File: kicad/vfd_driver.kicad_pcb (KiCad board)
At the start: 2 copper layers, 181.6 x 35.3 mm, 48 parts, among them CON1 AVR-ISP-6, J1 PWR, J2 Display, J6 MH, J7 MH, J8 MH, J9 MH, U1 ATTINY2313-20SU, U10 74HC595, U11 74HC595, U12 74HC595, U13 74HC595, U14 ULN2803A, U15 ULN2803A, U16 ULN2003, U17 ULN2003, U18 LM1117-3.3, U19 LT1073, U2 74HC595, U3 74HC595, U4 74HC595, U5 74HC595, U6 ULN2803A, U7 ULN2003, U8 ULN2003, U9 ULN2003

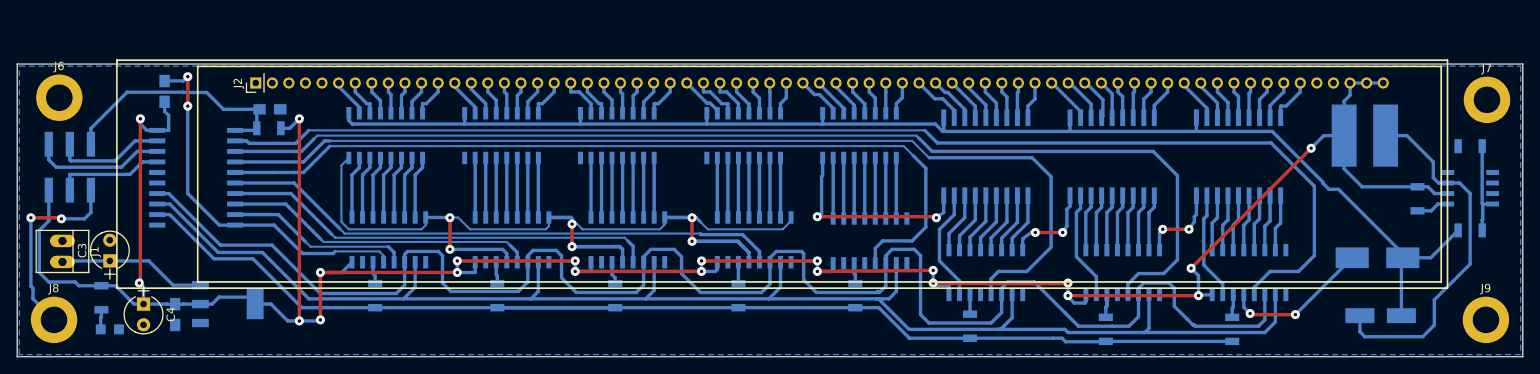
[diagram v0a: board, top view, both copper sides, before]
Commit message: routing
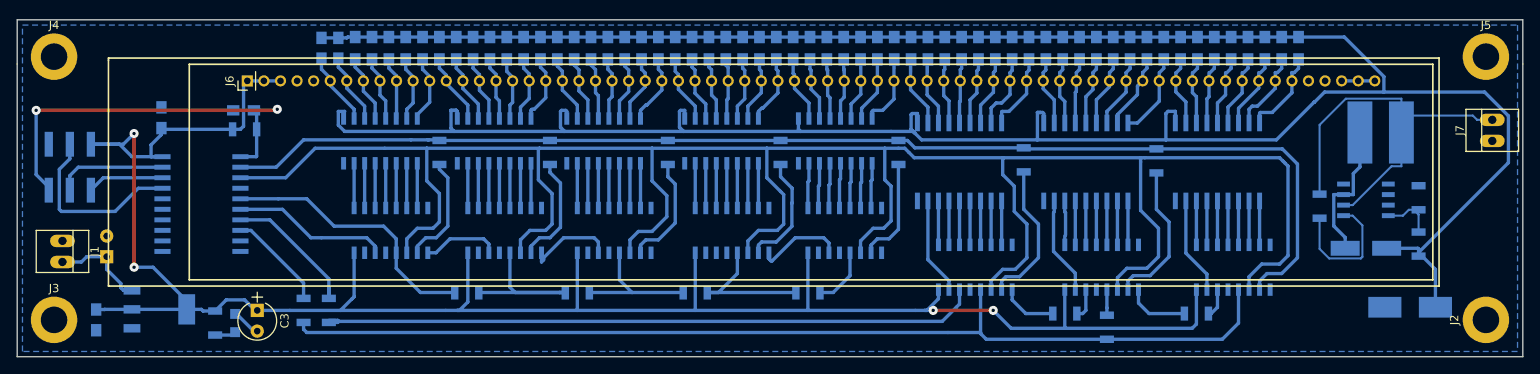
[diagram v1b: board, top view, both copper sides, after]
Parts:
- removed J8, J9: MH, Mounting_Holes:MountingHole_3.2mm_M3_DIN965_Pad
- removed U1: ATTINY2313-20SU, Housings_SOIC:SOIC-20W_7.5x12.8mm_Pitch1.27mm
- removed U2, U3, U4: 74HC595, Housings_SOIC:SOIC-16_3.9x9.9mm_Pitch1.27mm
- added J3: MH, Mounting_Holes:MountingHole_3.2mm_M3_DIN965_Pad, F.Cu at (19.1, 49.5)
- added J4: MH, Mounting_Holes:MountingHole_3.2mm_M3_DIN965_Pad, F.Cu at (19.1, 17.8)
- added J5: MH, Mounting_Holes:MountingHole_3.2mm_M3_DIN965_Pad, F.Cu at (191.8, 17.8)
- added R16: 1k, Resistors_SMD:R_0805_HandSoldering, B.Cu at (55.4, 16.8)
- added R17: 1k, Resistors_SMD:R_0805_HandSoldering, B.Cu at (57.4, 16.8)
- added R18: 1k, Resistors_SMD:R_0805_HandSoldering, B.Cu at (59.4, 16.8)
- added R19: 1k, Resistors_SMD:R_0805_HandSoldering, B.Cu at (61.5, 16.8)
- added R20: 1k, Resistors_SMD:R_0805_HandSoldering, B.Cu at (63.5, 16.8)
- added R21: 1k, Resistors_SMD:R_0805_HandSoldering, B.Cu at (65.5, 16.8)
- added R22: 1k, Resistors_SMD:R_0805_HandSoldering, B.Cu at (67.6, 16.8)
- added R23: 1k, Resistors_SMD:R_0805_HandSoldering, B.Cu at (69.6, 16.8)
- added R24: 1k, Resistors_SMD:R_0805_HandSoldering, B.Cu at (71.6, 16.8)
- added R25: 1k, Resistors_SMD:R_0805_HandSoldering, B.Cu at (73.7, 16.8)
- added R26: 1k, Resistors_SMD:R_0805_HandSoldering, B.Cu at (75.7, 16.8)
- added R27: 1k, Resistors_SMD:R_0805_HandSoldering, B.Cu at (77.7, 16.8)
- added R28: 1k, Resistors_SMD:R_0805_HandSoldering, B.Cu at (79.8, 16.8)
- added R29: 1k, Resistors_SMD:R_0805_HandSoldering, B.Cu at (81.8, 16.8)
- added R30: 1k, Resistors_SMD:R_0805_HandSoldering, B.Cu at (83.8, 16.8)
- added R31: 1k, Resistors_SMD:R_0805_HandSoldering, B.Cu at (85.9, 16.8)
- added R32: 1k, Resistors_SMD:R_0805_HandSoldering, B.Cu at (87.9, 16.8)
- added R33: 1k, Resistors_SMD:R_0805_HandSoldering, B.Cu at (89.9, 16.8)
- added R34: 1k, Resistors_SMD:R_0805_HandSoldering, B.Cu at (91.9, 16.8)
- added R35: 1k, Resistors_SMD:R_0805_HandSoldering, B.Cu at (94.0, 16.8)
- added R36: 1k, Resistors_SMD:R_0805_HandSoldering, B.Cu at (96.0, 16.8)
- added R37: 1k, Resistors_SMD:R_0805_HandSoldering, B.Cu at (98.0, 16.8)
- added R38: 1k, Resistors_SMD:R_0805_HandSoldering, B.Cu at (100.1, 16.8)
- added R39: 1k, Resistors_SMD:R_0805_HandSoldering, B.Cu at (102.1, 16.8)
- added R40: 1k, Resistors_SMD:R_0805_HandSoldering, B.Cu at (104.1, 16.8)
- added R41: 1k, Resistors_SMD:R_0805_HandSoldering, B.Cu at (106.2, 16.8)
- added R42: 1k, Resistors_SMD:R_0805_HandSoldering, B.Cu at (108.2, 16.8)
- added R43: 1k, Resistors_SMD:R_0805_HandSoldering, B.Cu at (110.2, 16.8)
- added R44: 1k, Resistors_SMD:R_0805_HandSoldering, B.Cu at (112.3, 16.8)
- added R45: 1k, Resistors_SMD:R_0805_HandSoldering, B.Cu at (114.3, 16.8)
- added R46: 1k, Resistors_SMD:R_0805_HandSoldering, B.Cu at (116.3, 16.8)
- added R47: 1k, Resistors_SMD:R_0805_HandSoldering, B.Cu at (118.4, 16.8)
- added R48: 1k, Resistors_SMD:R_0805_HandSoldering, B.Cu at (120.4, 16.8)
- added R49: 1k, Resistors_SMD:R_0805_HandSoldering, B.Cu at (122.4, 16.8)
- added R50: 1k, Resistors_SMD:R_0805_HandSoldering, B.Cu at (124.5, 16.8)
- added R51: 1k, Resistors_SMD:R_0805_HandSoldering, B.Cu at (126.5, 16.8)
- added R52: 1k, Resistors_SMD:R_0805_HandSoldering, B.Cu at (128.5, 16.8)
- added R53: 1k, Resistors_SMD:R_0805_HandSoldering, B.Cu at (130.6, 16.8)
- added R54: 1k, Resistors_SMD:R_0805_HandSoldering, B.Cu at (132.6, 16.8)
- added R55: 1k, Resistors_SMD:R_0805_HandSoldering, B.Cu at (134.6, 16.8)
- added R56: 1k, Resistors_SMD:R_0805_HandSoldering, B.Cu at (136.7, 16.8)
- added R57: 1k, Resistors_SMD:R_0805_HandSoldering, B.Cu at (138.7, 16.8)
- added R58: 1k, Resistors_SMD:R_0805_HandSoldering, B.Cu at (140.7, 16.8)
- added R59: 1k, Resistors_SMD:R_0805_HandSoldering, B.Cu at (142.7, 16.8)
- added R6: 1M, Resistors_SMD:R_1206, B.Cu at (183.6, 40.4)
- added R60: 1k, Resistors_SMD:R_0805_HandSoldering, B.Cu at (144.8, 16.8)
- added R61: 1k, Resistors_SMD:R_0805_HandSoldering, B.Cu at (146.8, 16.8)
- added R62: 1k, Resistors_SMD:R_0805_HandSoldering, B.Cu at (148.8, 16.8)
- added R63: 1k, Resistors_SMD:R_0805_HandSoldering, B.Cu at (150.9, 16.8)
- added R64: 1k, Resistors_SMD:R_0805_HandSoldering, B.Cu at (152.9, 16.8)
- added R65: 1k, Resistors_SMD:R_0805_HandSoldering, B.Cu at (154.9, 16.8)
- added R66: 1k, Resistors_SMD:R_0805_HandSoldering, B.Cu at (157.0, 16.8)
- added R67: 1k, Resistors_SMD:R_0805_HandSoldering, B.Cu at (159.0, 16.8)
- added R68: 1k, Resistors_SMD:R_0805_HandSoldering, B.Cu at (161.0, 16.8)
- added R69: 1k, Resistors_SMD:R_0805_HandSoldering, B.Cu at (163.1, 16.8)
- added R7: 4k7, Resistors_SMD:R_1206, B.Cu at (183.6, 34.8)
- added R70: 1k, Resistors_SMD:R_0805_HandSoldering, B.Cu at (165.1, 16.8)
- added R71: 1k, Resistors_SMD:R_0805_HandSoldering, B.Cu at (167.1, 16.8)
- added R72: 1k, Resistors_SMD:R_0805_HandSoldering, B.Cu at (169.2, 16.8)
- added R73: 0, Resistors_SMD:R_1206, B.Cu at (65.5, 29.3)
- added R74: 0, Resistors_SMD:R_1206, B.Cu at (78.9, 29.3)
- added R75: 0, Resistors_SMD:R_1206, B.Cu at (93.1, 29.3)
- added R76: 0, Resistors_SMD:R_1206, B.Cu at (106.7, 29.3)
- added R77: 0, Resistors_SMD:R_1206, B.Cu at (120.9, 29.3)
- added R78: 0, Resistors_SMD:R_1206, B.Cu at (136.0, 30.2)
- added R79: 0, Resistors_SMD:R_1206, B.Cu at (152.0, 30.4)
- added R80: 0, Resistors_SMD:R_1206, B.Cu at (146.1, 50.4)
- added U20: 74HC595, Housings_SOIC:SOIC-16_3.9x9.9mm_Pitch1.27mm, B.Cu at (145.4, 43.2)
- added U21: ULN2803A, Housings_SOIC:SOIC-18W_7.5x11.6mm_Pitch1.27mm, B.Cu at (143.5, 30.5)
- added U22: 74HC595, Housings_SOIC:SOIC-16_3.9x9.9mm_Pitch1.27mm, B.Cu at (161.3, 43.2)
- added U23: ULN2803A, Housings_SOIC:SOIC-18W_7.5x11.6mm_Pitch1.27mm, B.Cu at (159.4, 30.5)
- C2: value 100n -> 47µ; footprint Capacitors_SMD:C_0805_HandSoldering -> Capacitors_THT:CP_Radial_Tantal_D4.5mm_P2.50mm
- C4: value 47µ -> 100n; footprint Capacitors_THT:CP_Radial_Tantal_D4.5mm_P2.50mm -> Capacitors_SMD:C_0805_HandSoldering; moved to B.Cu
- D1: value 1N5818 -> LED; footprint Diodes_SMD:D_SMA_Handsoldering -> LEDs:LED_0805
- D2: value LED -> 1N5818; footprint LEDs:LED_0805 -> Diodes_SMD:D_SMA_Handsoldering
- J2: value Display -> MH; footprint modules:vfd_FUTABA_24-SD-01GK_24x1 -> Mounting_Holes:MountingHole_3.2mm_M3_DIN965_Pad
- J6: value MH -> Display; footprint Mounting_Holes:MountingHole_3.2mm_M3_DIN965_Pad -> modules:vfd_FUTABA_24-SD-01GK_24x1
- J7: value MH -> Step; footprint Mounting_Holes:MountingHole_3.2mm_M3_DIN965_Pad -> Connectors:PINHEAD1-2
- R1: value 10k -> 1k; footprint Resistors_SMD:R_1206 -> Capacitors_SMD:C_0805_HandSoldering
- R2: value 100 -> 1k; footprint Resistors_SMD:R_1206 -> Capacitors_SMD:C_0805_HandSoldering
- R3: value 1M -> 10k
- R4: value 4k7 -> 470
- R5: value 470 -> 100
- U11, U13: value 74HC595 -> ULN2003
- U14: value ULN2803A -> 74HC595; footprint Housings_SOIC:SOIC-18W_7.5x11.6mm_Pitch1.27mm -> Housings_SOIC:SOIC-16_3.9x9.9mm_Pitch1.27mm
- U15: value ULN2803A -> ULN2003; footprint Housings_SOIC:SOIC-18W_7.5x11.6mm_Pitch1.27mm -> Housings_SOIC:SOIC-16_3.9x9.9mm_Pitch1.27mm
- U16, U8: value ULN2003 -> 74HC595
- U18: value LM1117-3.3 -> 74HC595; footprint modules:SOT-223_pin4_3 -> Housings_SOIC:SOIC-16_3.9x9.9mm_Pitch1.27mm
- U19: value LT1073 -> ULN2803A; footprint Housings_SOIC:SOIC-8_3.9x4.9mm_Pitch1.27mm -> Housings_SOIC:SOIC-18W_7.5x11.6mm_Pitch1.27mm
- U5: value 74HC595 -> LM1117-3.3; footprint Housings_SOIC:SOIC-16_3.9x9.9mm_Pitch1.27mm -> modules:SOT-223_pin4_3
- U6: value ULN2803A -> ATTINY2313-20SU; footprint Housings_SOIC:SOIC-18W_7.5x11.6mm_Pitch1.27mm -> Housings_SOIC:SOIC-20W_7.5x12.8mm_Pitch1.27mm
- U7: value ULN2003 -> LT1073; footprint Housings_SOIC:SOIC-16_3.9x9.9mm_Pitch1.27mm -> Housings_SOIC:SOIC-8_3.9x4.9mm_Pitch1.27mm
- moved R4 152.9 mm to (38.5, 49.9), turned to 270 degrees
- moved D2 151.8 mm to (177.3, 40.9)
- moved R3 148.3 mm to (42.0, 26.5)
- moved R5 147.4 mm to (171.7, 35.8)
- moved D1 138.2 mm to (40.9, 49.9), turned to 270 degrees
- moved R2 131.4 mm to (53.3, 16.8)
- moved U7 118.5 mm to (177.3, 35.1), turned to 0 degrees
- moved R13 109.0 mm to (52.2, 48.4), turned to 90 degrees
- moved U6 94.8 mm to (36.8, 35.6), turned to 180 degrees
- moved U11 92.4 mm to (72.1, 27.9), turned to 90 degrees
- moved J6 90.7 mm to (110.4, 20.7), turned to 90 degrees
- moved U18 90.3 mm to (130.2, 43.2), turned to 270 degrees
- moved J2 85.3 mm to (191.8, 49.5)
- moved R8 80.4 mm to (49.1, 48.4)
- moved U10 74.7 mm to (73.4, 38.7)
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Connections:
- C2 pad 1: GND -> Net-(C2-Pad1)
- C2 pad 2: VCC -> GND
- C3 pad 1: Net-(C3-Pad1) -> VCC
- C4 pad 1: VCC -> GND
- C4 pad 2: GND -> VCC
- D1 pad 1: +36V -> GND
- D2 pad 1: GND -> +36V
- J1 pad 2: Net-(C3-Pad1) -> Net-(C2-Pad1)
- J6 pad 1: GND -> VCC
- L1 pad 1: VCC -> Net-(J7-Pad2)
- L1 pad 2: Net-(D1-Pad2) -> Net-(D2-Pad2)
- R1 pad 1: VCC -> +36V
- R1 pad 2: /reset -> /Sheet59FF2CCC/L1_1
- R10 pad 1: Net-(R10-Pad1) -> /Sheet5A12BB8F/RCLK
- R10 pad 2: /SER -> /Sheet5A11F95F/RCLK
- R11 pad 1: Net-(R11-Pad1) -> /Sheet5A11F95F/RCLK
- R11 pad 2: /SER -> /Sheet5A12BB9F/RCLK
- R12 pad 1: Net-(R12-Pad1) -> /Sheet5A12BB9F/RCLK
- R12 pad 2: /SER -> /Sheet5A12BBAF/RCLK
- R13 pad 2: /SER -> /SER_POS
- R14 pad 1: Net-(R14-Pad1) -> /Sheet5A13BBCF/SER
- R14 pad 2: /SER -> /Sheet5A13BBAF/SER_OUT
- R15 pad 1: Net-(R15-Pad1) -> /Sheet5A13BBBF/SER
- R15 pad 2: /SER -> /Sheet5A13BBCF/SER_OUT
- R2 pad 1: VCC -> +36V
- R2 pad 2: Net-(R2-Pad2) -> /Sheet59FF2CCC/L1_2
- R3 pad 1: +36V -> VCC
- R3 pad 2: Net-(R3-Pad2) -> /reset
- R4 pad 1: Net-(R3-Pad2) -> VCC
- R4 pad 2: GND -> Net-(D1-Pad2)
- R5 pad 1: VCC -> Net-(J7-Pad2)
- R5 pad 2: Net-(D2-Pad2) -> Net-(R5-Pad2)
- R8 pad 1: Net-(R8-Pad1) -> /RCLK_0
- R8 pad 2: /SER -> /Sheet5A13BBAF/RCLK
- R9 pad 1: Net-(R9-Pad1) -> /RCLK_7
- R9 pad 2: /SER -> /Sheet5A12BB8F/RCLK
- U10 pad 10: /SRCLR -> Net-(R74-Pad1)
- U10 pad 12: /RCLK_1 -> /Sheet5A12BB8F/RCLK
- U10 pad 14: Net-(R12-Pad1) -> /Sheet5A12BB8F/SER
- U10 pad 15: Net-(U10-Pad15) -> (no net)
- U10 pad 9: (no net) -> /Sheet5A11F95F/SER
- U11 pad 1: Net-(U11-Pad1) -> Net-(U10-Pad7)
- U11 pad 10: /SRCLR -> /Sheet59FF2CCC/L2_1
- U11 pad 11: /SRCLK -> /Sheet59FF2CCC/L2_2
- U11 pad 12: /RCLK_2 -> /Sheet59FF2CCC/L2_3
- U11 pad 13: GND -> /Sheet59FF2CCC/L2_4
- U11 pad 14: Net-(R13-Pad1) -> /Sheet59FF2CCC/L2_5
- U11 pad 15: Net-(U11-Pad15) -> /Sheet59FF2CCC/L2_6
- U11 pad 16: VCC -> /Sheet59FF2CCC/L2_7
- U11 pad 2: Net-(U11-Pad2) -> Net-(U10-Pad6)
- U11 pad 3: Net-(U11-Pad3) -> Net-(U10-Pad5)
- U11 pad 4: Net-(U11-Pad4) -> Net-(U10-Pad4)
- U11 pad 5: Net-(U11-Pad5) -> Net-(U10-Pad3)
- U11 pad 6: Net-(U11-Pad6) -> Net-(U10-Pad2)
- U11 pad 7: Net-(U11-Pad7) -> Net-(U10-Pad1)
- U11 pad 9: (no net) -> +36V
- U12 pad 10: /SRCLR -> Net-(R75-Pad1)
- U12 pad 12: /RCLK_5 -> /Sheet5A11F95F/RCLK
- U12 pad 14: Net-(R14-Pad1) -> /Sheet5A11F95F/SER
- U12 pad 9: (no net) -> /Sheet5A12BB9F/SER
- U13 pad 1: Net-(U13-Pad1) -> Net-(U12-Pad7)
- U13 pad 10: /SRCLR -> /Sheet59FF2CCC/L3_1
- U13 pad 11: /SRCLK -> /Sheet59FF2CCC/L3_2
- U13 pad 12: /RCLK_7 -> /Sheet59FF2CCC/L3_3
- U13 pad 13: GND -> /Sheet59FF2CCC/L3_4
- U13 pad 14: Net-(R15-Pad1) -> /Sheet59FF2CCC/L3_5
- U13 pad 15: (no net) -> /Sheet59FF2CCC/L3_6
- U13 pad 16: VCC -> /Sheet59FF2CCC/L3_7
- U13 pad 2: Net-(U13-Pad2) -> Net-(U12-Pad6)
- U13 pad 3: Net-(U13-Pad3) -> Net-(U12-Pad5)
- U13 pad 4: Net-(U13-Pad4) -> Net-(U12-Pad4)
- U13 pad 5: Net-(U13-Pad5) -> Net-(U12-Pad3)
- U13 pad 6: Net-(U13-Pad6) -> Net-(U12-Pad2)
- U13 pad 7: Net-(U13-Pad7) -> Net-(U12-Pad1)
- U13 pad 9: (no net) -> +36V
- U14 pad 1: Net-(U10-Pad7) -> Net-(U14-Pad1)
- U14 pad 10: +36V -> Net-(R76-Pad1)
- U14 pad 11: /G21 -> /SRCLK
- U14 pad 12: /G22 -> /Sheet5A12BB9F/RCLK
- U14 pad 13: /G23 -> GND
- U14 pad 14: /G24 -> /Sheet5A12BB9F/SER
- U14 pad 15: /G25 -> (no net)
- U14 pad 16: /G26 -> VCC
- U14 pad 2: Net-(U10-Pad6) -> Net-(U14-Pad2)
- U14 pad 3: Net-(U10-Pad5) -> Net-(U14-Pad3)
- U14 pad 4: Net-(U10-Pad4) -> Net-(U14-Pad4)
- U14 pad 5: Net-(U10-Pad3) -> Net-(U14-Pad5)
- U14 pad 6: Net-(U10-Pad2) -> Net-(U14-Pad6)
- U14 pad 7: Net-(U10-Pad1) -> Net-(U14-Pad7)
- U14 pad 8: Net-(U10-Pad15) -> GND
- U14 pad 9: GND -> /Sheet5A12BBAF/SER
- U15 pad 1: Net-(U11-Pad7) -> Net-(U14-Pad7)
- U15 pad 10: +36V -> /Sheet59FF2CCC/L4_1
- U15 pad 11: /G31 -> /Sheet59FF2CCC/L4_2
- U15 pad 12: /G32 -> /Sheet59FF2CCC/L4_3
- U15 pad 13: /G33 -> /Sheet59FF2CCC/L4_4
- U15 pad 14: /G34 -> /Sheet59FF2CCC/L4_5
- U15 pad 15: /G35 -> /Sheet59FF2CCC/L4_6
- U15 pad 16: /G36 -> /Sheet59FF2CCC/L4_7
- U15 pad 2: Net-(U11-Pad6) -> Net-(U14-Pad6)
- U15 pad 3: Net-(U11-Pad5) -> Net-(U14-Pad5)
- U15 pad 4: Net-(U11-Pad4) -> Net-(U14-Pad4)
- U15 pad 5: Net-(U11-Pad3) -> Net-(U14-Pad3)
- U15 pad 6: Net-(U11-Pad2) -> Net-(U14-Pad2)
- U15 pad 7: Net-(U11-Pad1) -> Net-(U14-Pad1)
- U15 pad 8: Net-(U11-Pad15) -> GND
- U15 pad 9: GND -> +36V
- U16 pad 1: Net-(U12-Pad7) -> Net-(U16-Pad1)
- U16 pad 10: /L31 -> Net-(R77-Pad1)
- U16 pad 11: /L32 -> /SRCLK
- U16 pad 12: /L33 -> /Sheet5A12BBAF/RCLK
- U16 pad 13: /L34 -> GND
- U16 pad 14: /L35 -> /Sheet5A12BBAF/SER
- U16 pad 15: /L36 -> (no net)
- U16 pad 16: /L37 -> VCC
- U16 pad 2: Net-(U12-Pad6) -> Net-(U16-Pad2)
- U16 pad 3: Net-(U12-Pad5) -> Net-(U16-Pad3)
- U16 pad 4: Net-(U12-Pad4) -> Net-(U16-Pad4)
- U16 pad 5: Net-(U12-Pad3) -> Net-(U16-Pad5)
- U16 pad 6: Net-(U12-Pad2) -> Net-(U16-Pad6)
- U16 pad 7: Net-(U12-Pad1) -> Net-(U16-Pad7)
- U16 pad 9: +36V -> (no net)
- U17 pad 1: Net-(U13-Pad7) -> Net-(U16-Pad7)
- U17 pad 10: /L51 -> /Sheet59FF2CCC/L5_1
- U17 pad 11: /L52 -> /Sheet59FF2CCC/L5_2
- U17 pad 12: /L53 -> /Sheet59FF2CCC/L5_3
- U17 pad 13: /L54 -> /Sheet59FF2CCC/L5_4
- U17 pad 14: /L55 -> /Sheet59FF2CCC/L5_5
- U17 pad 15: /L56 -> /Sheet59FF2CCC/L5_6
- U17 pad 16: /L57 -> /Sheet59FF2CCC/L5_7
- U17 pad 2: Net-(U13-Pad6) -> Net-(U16-Pad6)
- U17 pad 3: Net-(U13-Pad5) -> Net-(U16-Pad5)
- U17 pad 4: Net-(U13-Pad4) -> Net-(U16-Pad4)
- U17 pad 5: Net-(U13-Pad3) -> Net-(U16-Pad3)
- U17 pad 6: Net-(U13-Pad2) -> Net-(U16-Pad2)
- U17 pad 7: Net-(U13-Pad1) -> Net-(U16-Pad1)
- U18 pad 1: GND -> Net-(U18-Pad1)
- U18 pad 2: VCC -> Net-(U18-Pad2)
- U18 pad 3: Net-(C3-Pad1) -> Net-(U18-Pad3)
- U19 pad 1: Net-(R2-Pad2) -> Net-(U18-Pad7)
- U19 pad 2: VCC -> Net-(U18-Pad6)
- U19 pad 3: Net-(D1-Pad2) -> Net-(U18-Pad5)
- U19 pad 4: GND -> Net-(U18-Pad4)
- U19 pad 5: GND -> Net-(U18-Pad3)
- U19 pad 6: (no net) -> Net-(U18-Pad2)
- U19 pad 7: (no net) -> Net-(U18-Pad1)
- U19 pad 8: Net-(R3-Pad2) -> Net-(U18-Pad15)
- U5 pad 1: Net-(U5-Pad1) -> GND
- U5 pad 2: Net-(U5-Pad2) -> VCC
- U5 pad 3: Net-(U5-Pad3) -> Net-(C2-Pad1)
- U6 pad 1: Net-(U2-Pad7) -> /reset
- U6 pad 10: +36V -> GND
- U6 pad 11: /G11 -> (no net)
- U6 pad 12: /G12 -> (no net)
- U6 pad 13: /G13 -> (no net)
- U6 pad 14: /G14 -> (no net)
- U6 pad 15: /G15 -> (no net)
- U6 pad 16: /G16 -> (no net)
- U6 pad 17: /G17 -> /MOSI
- U6 pad 18: /G18 -> /MISO
- U6 pad 2: Net-(U2-Pad6) -> /SRCLR
- U6 pad 3: Net-(U2-Pad5) -> /SRCLK
- U6 pad 4: Net-(U2-Pad4) -> (no net)
- U6 pad 5: Net-(U2-Pad3) -> /RCLK_7
- U6 pad 6: Net-(U2-Pad2) -> /SER_DAT
- U6 pad 7: Net-(U2-Pad1) -> /SER_POS
- U6 pad 8: Net-(U2-Pad15) -> /RCLK_0
- U6 pad 9: GND -> (no net)
- U7 pad 1: Net-(U3-Pad7) -> Net-(R5-Pad2)
- U7 pad 2: Net-(U3-Pad6) -> Net-(J7-Pad2)
- U7 pad 3: Net-(U3-Pad5) -> Net-(D2-Pad2)
- U7 pad 4: Net-(U3-Pad4) -> GND
- U7 pad 5: Net-(U3-Pad3) -> GND
- U7 pad 6: Net-(U3-Pad2) -> (no net)
- U7 pad 7: Net-(U3-Pad1) -> (no net)
- U7 pad 8: GND -> Net-(R6-Pad2)
- U8 pad 1: Net-(U4-Pad7) -> Net-(U8-Pad1)
- U8 pad 10: /L21 -> Net-(R73-Pad1)
- U8 pad 11: /L22 -> /SRCLK
- U8 pad 12: /L23 -> /RCLK_7
- U8 pad 13: /L24 -> GND
- U8 pad 14: /L25 -> /SER_DAT
- U8 pad 15: /L26 -> (no net)
- U8 pad 16: /L27 -> VCC
- U8 pad 2: Net-(U4-Pad6) -> Net-(U8-Pad2)
- U8 pad 3: Net-(U4-Pad5) -> Net-(U8-Pad3)
- U8 pad 4: Net-(U4-Pad4) -> Net-(U8-Pad4)
- U8 pad 5: Net-(U4-Pad3) -> Net-(U8-Pad5)
- U8 pad 6: Net-(U4-Pad2) -> Net-(U8-Pad6)
- U8 pad 7: Net-(U4-Pad1) -> Net-(U8-Pad7)
- U8 pad 9: +36V -> /Sheet5A12BB8F/SER
- U9 pad 1: Net-(U5-Pad7) -> Net-(U8-Pad7)
- U9 pad 10: /L47 -> /Sheet59FF2CCC/L1_1
- U9 pad 11: /L46 -> /Sheet59FF2CCC/L1_2
- U9 pad 12: /L45 -> /Sheet59FF2CCC/L1_3
- U9 pad 13: /L44 -> /Sheet59FF2CCC/L1_4
- U9 pad 14: /L43 -> /Sheet59FF2CCC/L1_5
- U9 pad 15: /L42 -> /Sheet59FF2CCC/L1_6
- U9 pad 16: /L41 -> /Sheet59FF2CCC/L1_7
- U9 pad 2: Net-(U5-Pad6) -> Net-(U8-Pad6)
- U9 pad 3: Net-(U5-Pad5) -> Net-(U8-Pad5)
- U9 pad 4: Net-(U5-Pad4) -> Net-(U8-Pad4)
- U9 pad 5: Net-(U5-Pad3) -> Net-(U8-Pad3)
- U9 pad 6: Net-(U5-Pad2) -> Net-(U8-Pad2)
- U9 pad 7: Net-(U5-Pad1) -> Net-(U8-Pad1)
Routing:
- net GND: track 263.7 -> 11.2 mm, vias 18 -> 0
- net +36V: track 161.6 -> 347.3 mm
- net /RCLK_2: track 151.9 -> 0.00 mm
- net /SER: track 150.3 -> 0.00 mm
- net /RCLK_1: track 135.1 -> 0.00 mm
- net /Sheet5A13BBAF/RCLK: track 0.00 -> 124.2 mm
- net /RCLK_0: track 120.5 -> 12.1 mm
- net Net-(R13-Pad1): track 2.94 -> 80.0 mm
- net /RCLK_6: track 69.5 -> 0.00 mm
- net /RCLK_7: track 102.1 -> 32.6 mm
- net /SRCLK: track 199.8 -> 267.1 mm
- net VCC: track 309.4 -> 250.1 mm, vias 21 -> 4
- net /RCLK_5: track 52.7 -> 0.00 mm
- net Net-(J7-Pad2): track 0.00 -> 47.8 mm
- net Net-(D1-Pad2): track 43.6 -> 2.56 mm
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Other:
- board size 181.6 x 35.3 mm -> 181.6 x 40.6 mm
